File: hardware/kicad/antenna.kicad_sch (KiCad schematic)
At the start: 10 parts, among them J5 BWIPX-1-001E, J7 BWIPX-1-001E, U15 SKY13414-485LF, U16 SKY13414-485LF

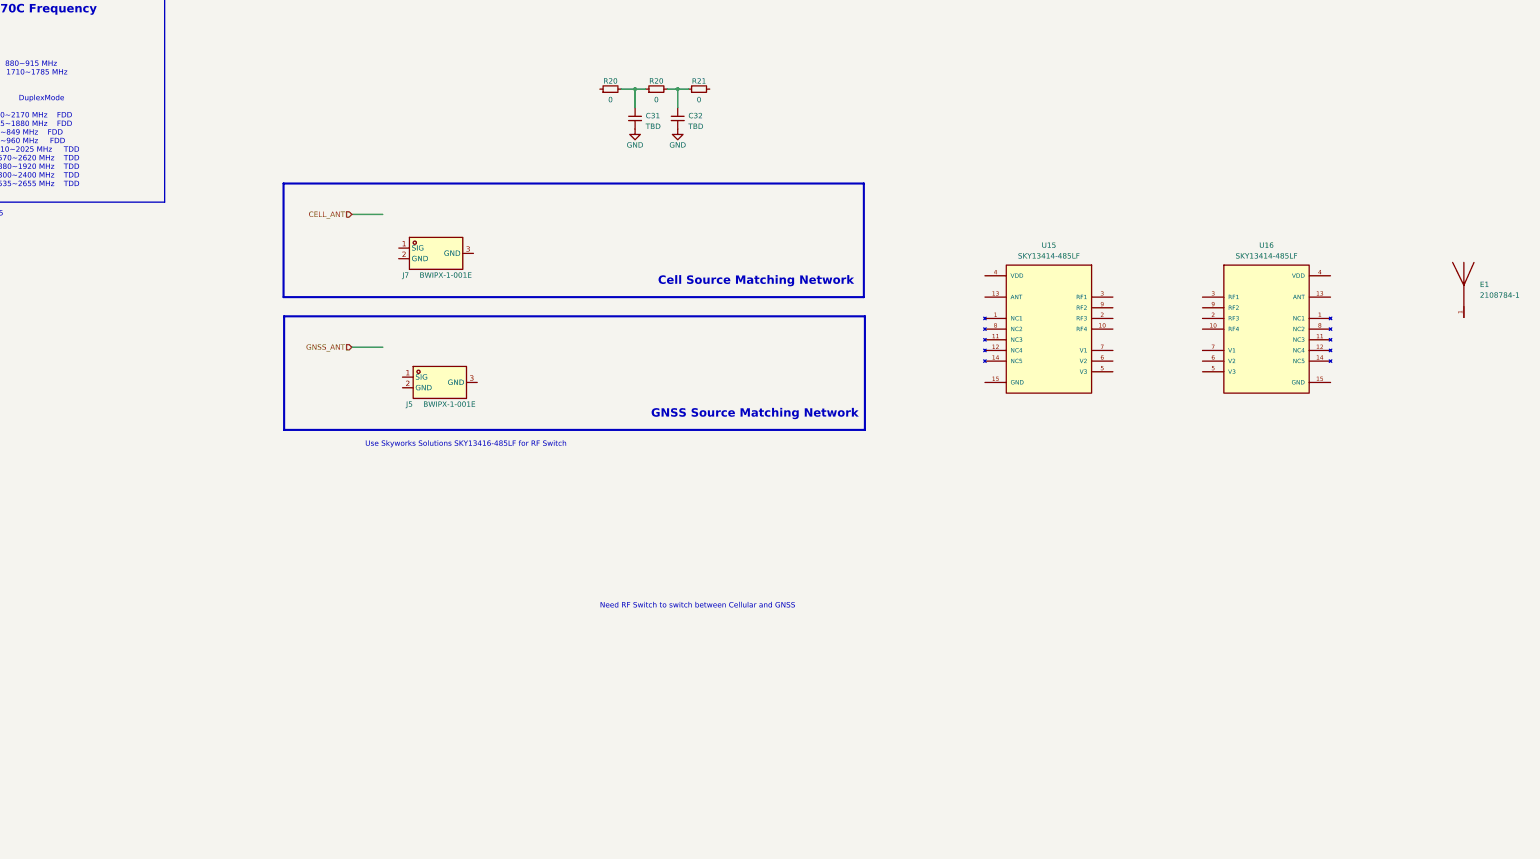
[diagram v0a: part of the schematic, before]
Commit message: update antenna
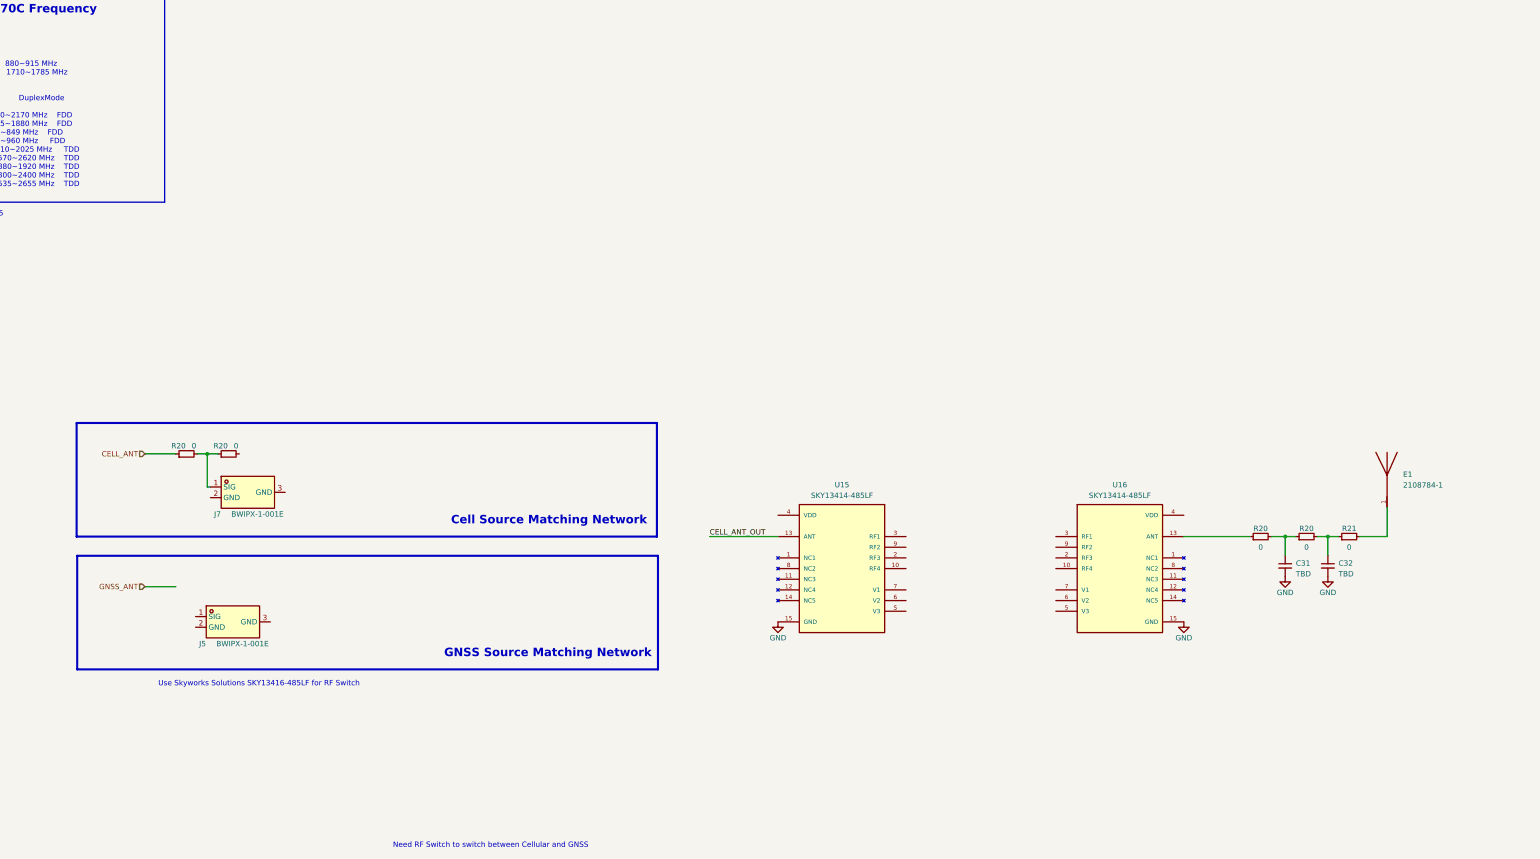
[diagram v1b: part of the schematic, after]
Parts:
- added R20 (x2): 0, Resistor_SMD:R_0402_1005Metric, symbol Device:R_Small
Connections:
- net CELL_ANT: now also R20.1
- net GND: now also U15.15 (GND), U16.15 (GND)
- net at R20.1: now also U16.13 (ANT)
- net at J7.1 (SIG): now also R20.1, R20.2
- net at E1.1: now also R21.2
- net CELL_ANT_OUT: now reaches U15.13 (ANT)
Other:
- moved on the sheet: C31, C32, E1, J5, J7, R20, R21, U15, U16
